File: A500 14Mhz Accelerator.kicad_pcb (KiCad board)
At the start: 2 copper layers, 121.9 x 57.1 mm, 26 parts, among them J1 Speed Selector, U1 68000 Boardside, U10 74HC74, U2 68HC000 Socket, U3 74HC86, U4 74HC74, U5 74LS27, U6 74LS112, U7 74HC04, U8 74LS157, U9 74LS157

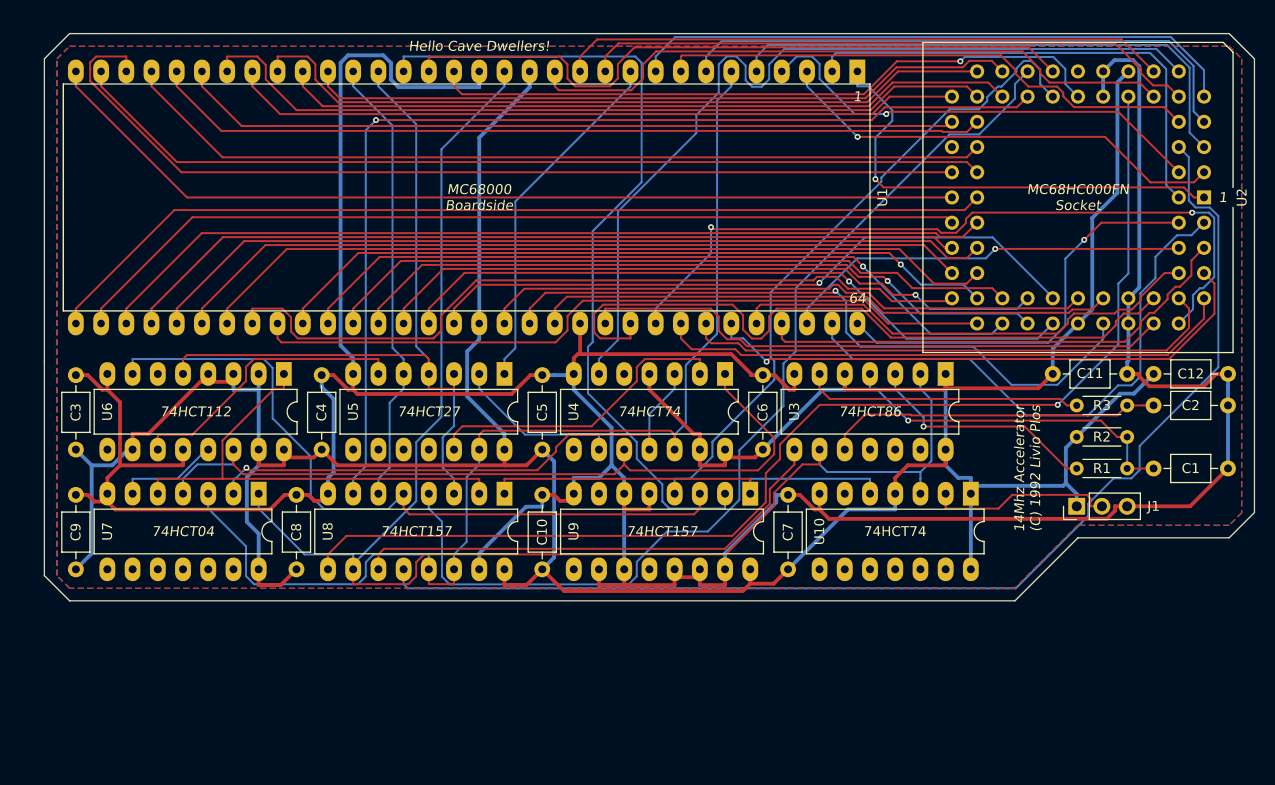
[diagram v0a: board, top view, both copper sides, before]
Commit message: Add files via upload
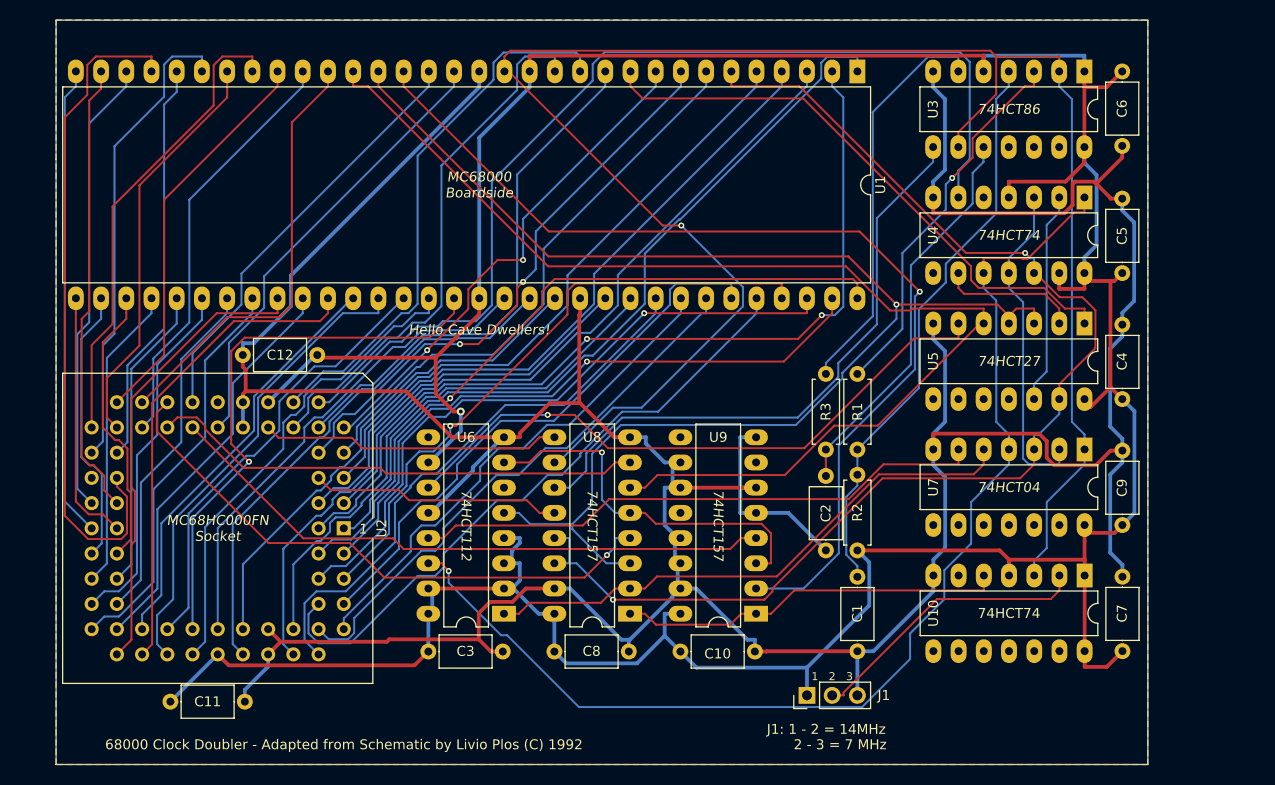
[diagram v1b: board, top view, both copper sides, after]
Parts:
- C1, C10, C11, C12, C2, C3, C4, C5, C6, C7, C8, C9: footprint Capacitor_THT:C_Axial_L3.8mm_D2.6mm_P7.50mm_Horizontal -> Capacitor_THT:C_Axial_L5.1mm_D3.1mm_P7.50mm_Horizontal
- R1, R2, R3: footprint Resistor_THT:R_Axial_DIN0204_L3.6mm_D1.6mm_P5.08mm_Horizontal -> Resistor_THT:R_Axial_DIN0207_L6.3mm_D2.5mm_P7.62mm_Horizontal
- U1: footprint Package_DIP:DIP-64_W25.4mm_SIL_Headers -> Package_DIP:DIP-64_W22.86mm_LongPads
- moved C9 105.5 mm to (192.4, 135.9)
- moved C11 94.8 mm to (96.5, 153.7)
- moved U2 92.9 mm to (114.0, 136.2)
- moved C12 84.3 mm to (111.3, 118.7), turned to 180 degrees
- moved U7 83.3 mm to (188.6, 128.3)
- moved C4 80.8 mm to (192.4, 123.2)
- moved C5 61.1 mm to (192.4, 110.5)
- moved U5 58.7 mm to (188.6, 115.6)
- moved C6 52.6 mm to (192.4, 90.2), turned to 270 degrees
- moved C2 43.1 mm to (162.6, 138.4), turned to 90 degrees
- moved C1 41.6 mm to (165.7, 148.6), turned to 90 degrees
- moved C3 40.9 mm to (122.5, 148.6), turned to 0 degrees
- moved U4 40.3 mm to (188.6, 102.9)
- moved U1 40.2 mm to (165.7, 90.2)
- moved C7 34.7 mm to (192.4, 148.6)
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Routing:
- net /CPU_AS14: track 119.8 -> 25.2 mm
- net /CPU_CLK14: track 117.8 -> 30.2 mm, vias 1 -> 0
- net /CPU_VPA: track 45.7 -> 118.6 mm
- net /CPU_A5: track 96.9 -> 25.7 mm
- net /CPU_A6: track 91.3 -> 28.0 mm
- net /CPU_A7: track 91.1 -> 28.7 mm
- net /CPU_E: track 79.2 -> 140.8 mm, vias 0 -> 1
- net /CPU_A9: track 86.1 -> 30.8 mm
- net /CPU_VPA14: track 105.2 -> 50.0 mm, vias 1 -> 0
- net /CPU_A8: track 85.6 -> 30.8 mm
- net /CPU_A2: track 97.9 -> 46.1 mm
- net /A500 14Mhz Accelerator Sheet 2/_E_OUT: track 10.3 -> 58.0 mm
- net /CPU_A3: track 93.4 -> 46.0 mm
- net /CPU_A4: track 94.4 -> 47.6 mm
- net /CPU_A11: track 81.4 -> 35.4 mm
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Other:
- board size 121.9 x 57.1 mm -> 110 x 75 mm
- board text added: "1 2 3"
- board text added: "2 - 3 = 7 MHz"
- board text added: "68000 Clock Doubler - Adapted from Schematic by Livio Plos (C) 1992"
- board text added: "J1: 1 - 2 = 14MHz"
- board text removed: "14Mhz Accelerator (C) 1992 Livio Plos"
